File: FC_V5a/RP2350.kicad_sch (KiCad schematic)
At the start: 29 parts, among them SW4 SW_Push, U11 W25Q128JVS, U18 RP2350_60QFN, Y1 ABM8-272-T3

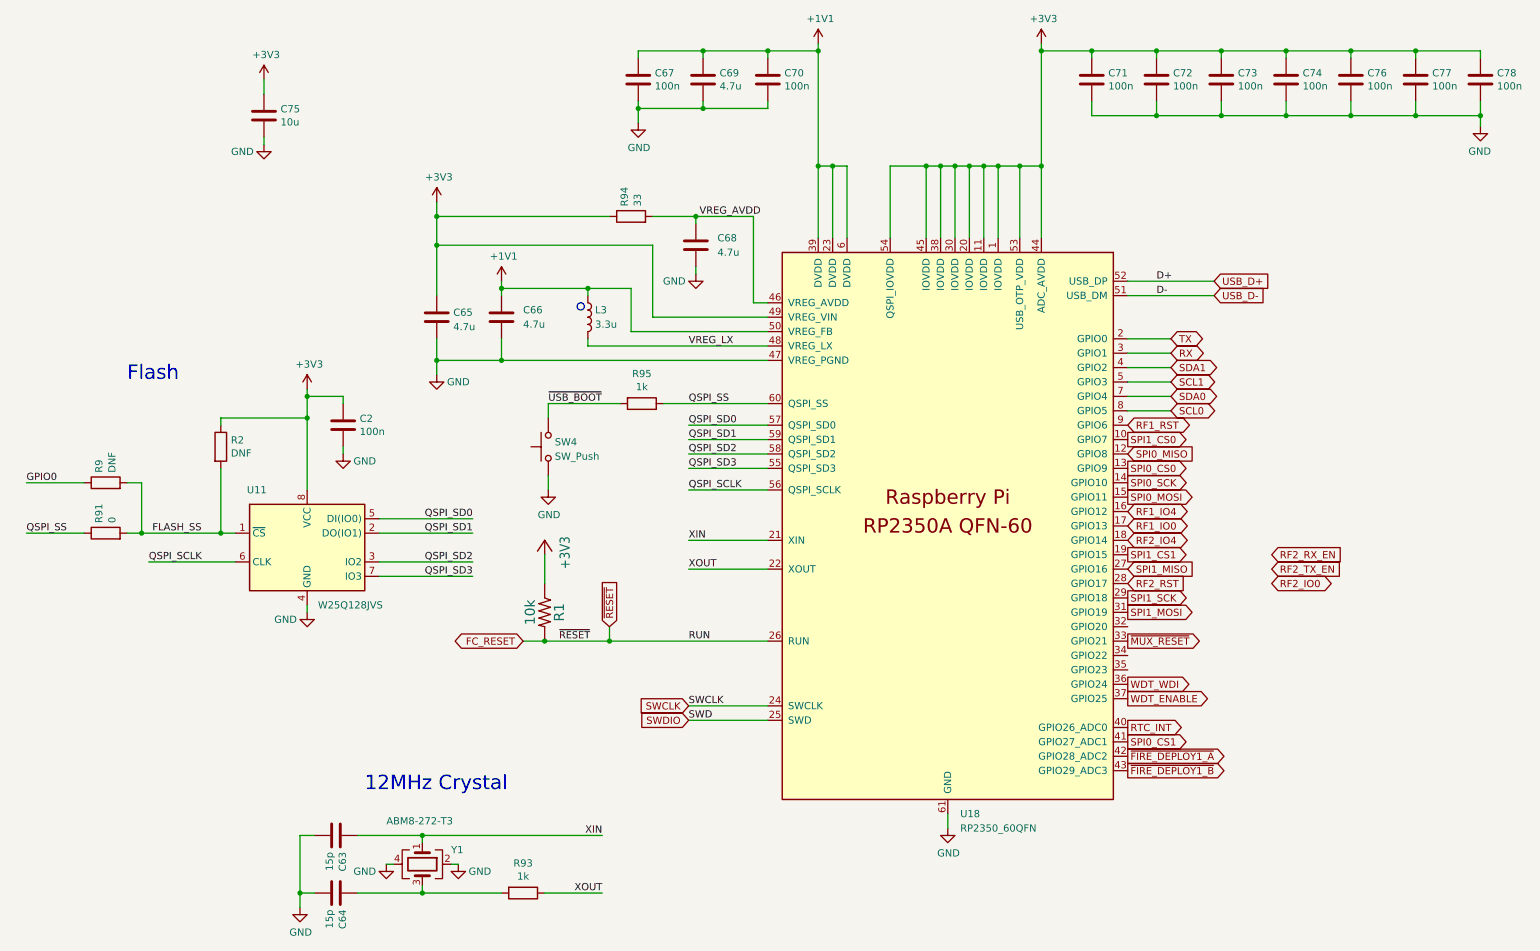
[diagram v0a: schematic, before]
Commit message: Initial V5a Layout Complete
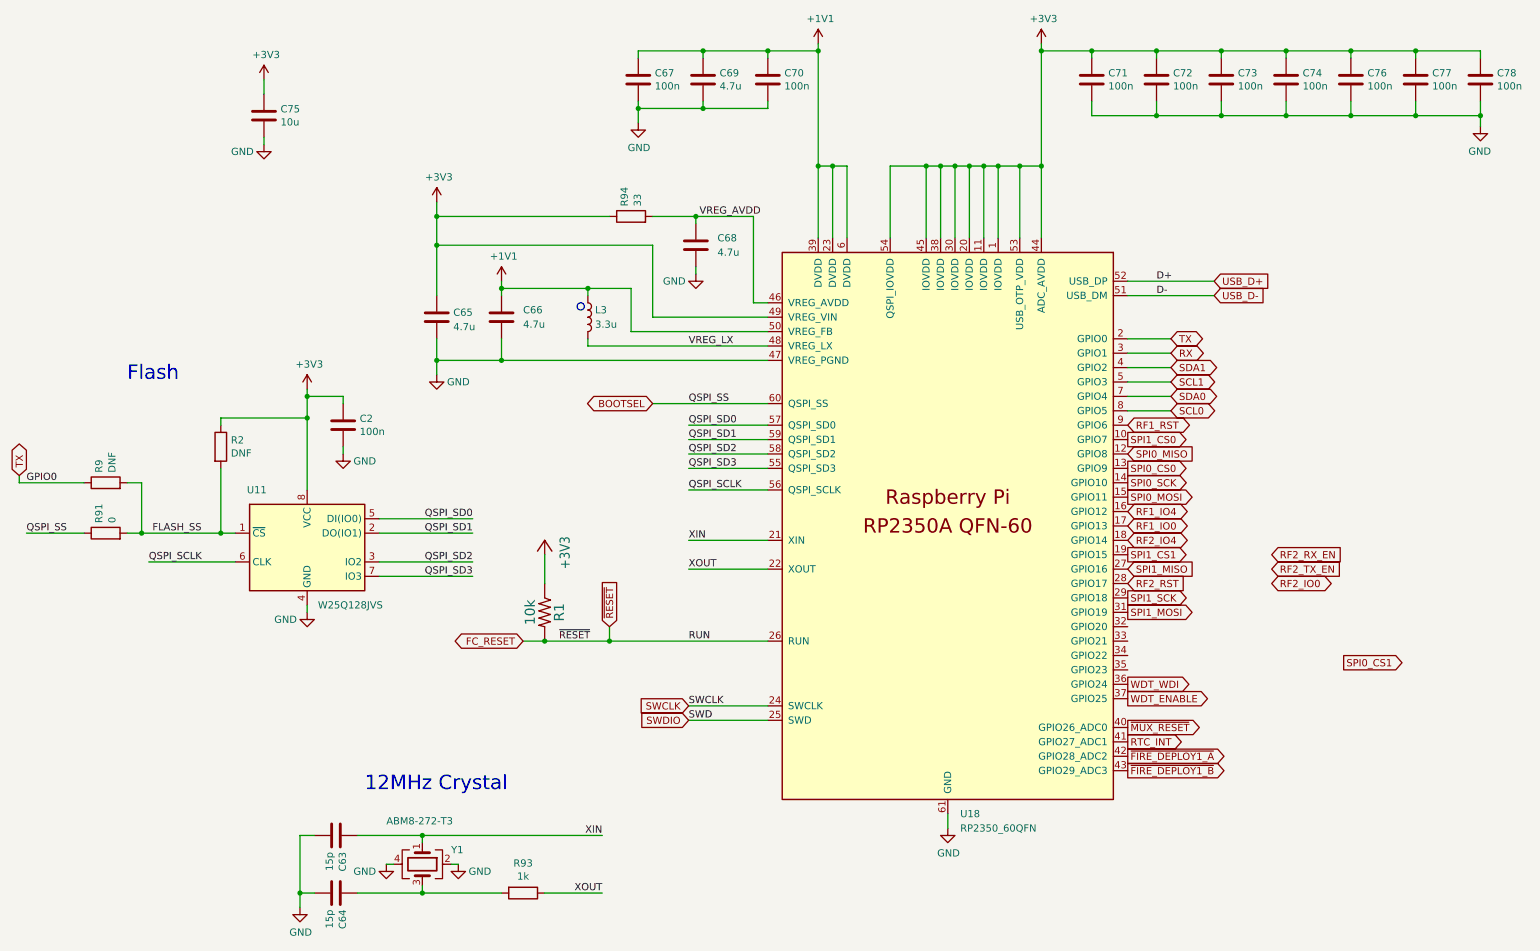
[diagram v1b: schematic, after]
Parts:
- removed R95: 1k, Resistor_SMD:R_0402_1005Metric, symbol Device:R
- removed SW4: SW_Push, Button_Switch_SMD:SW_Push_1P1T_NO_Vertical_Wuerth_434133025816, symbol Switch:SW_Push
- U11: footprint Package_SO:SOIC-8_5.23x5.23mm_P1.27mm -> Package_SO:SOIC-8_5.3x5.3mm_P1.27mm
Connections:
- net GPIO0 is gone; now on net TX: R9.1
- net RTC_INT: now also U18.41 (GPIO27_ADC1); no longer U18.40 (GPIO26_ADC0)
- net SPI0_CS1: no longer U18.41 (GPIO27_ADC1)
- net ~{MUX_RESET}: now also U18.40 (GPIO26_ADC0); no longer U18.33 (GPIO21)
- net QSPI_SS renamed BOOTSEL

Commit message: Initial DRC Errors Cleaned Up
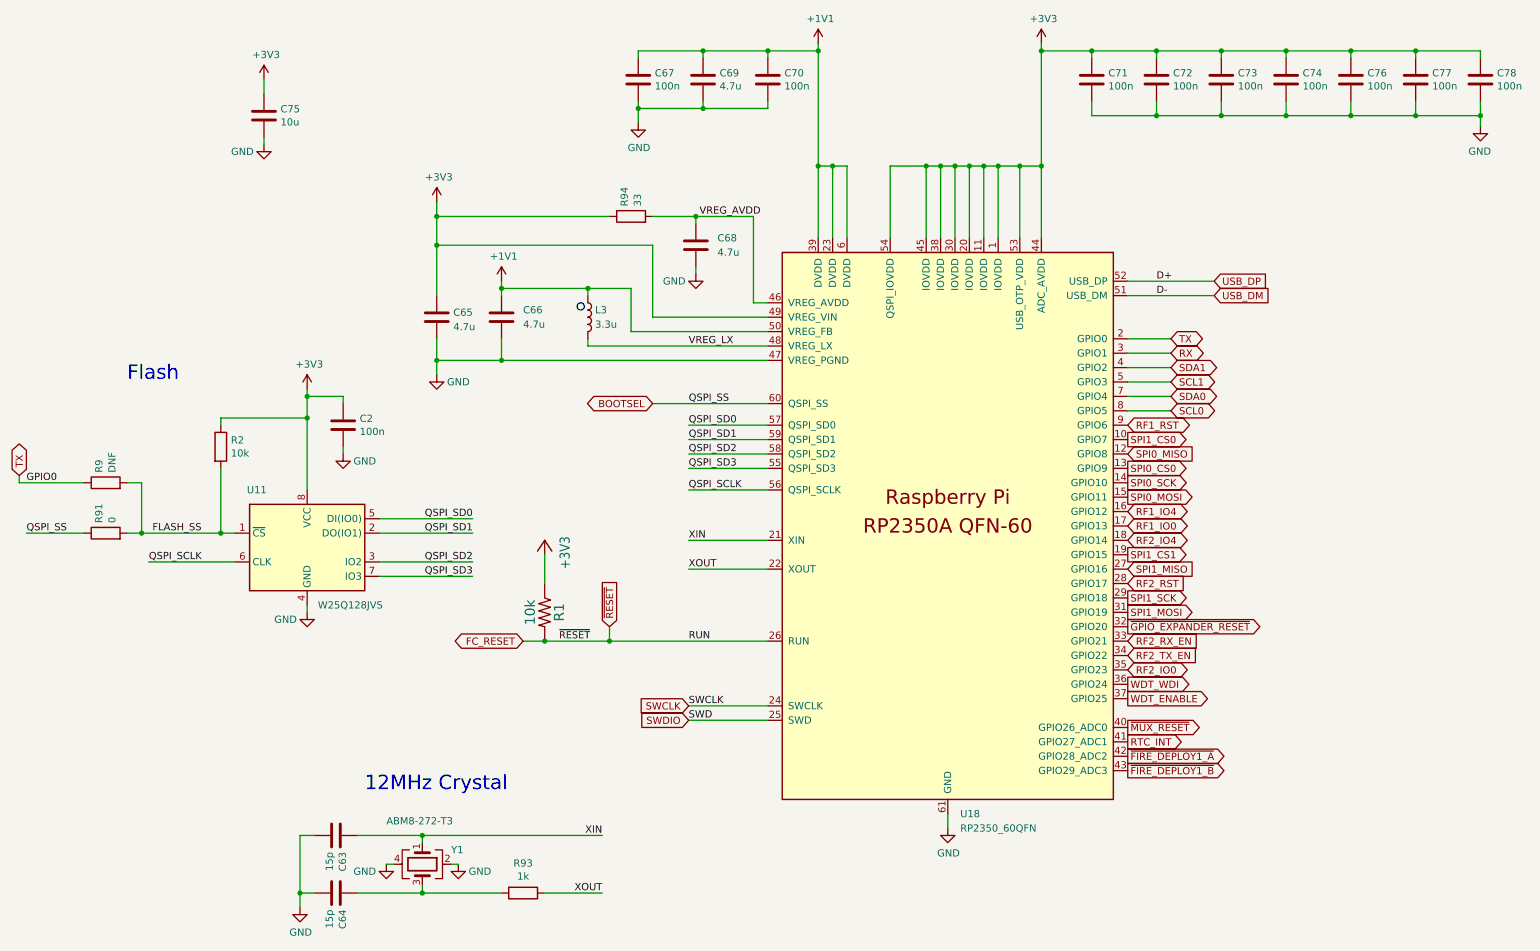
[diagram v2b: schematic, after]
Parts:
- R2: value DNF -> 10k
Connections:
- net RF2_IO0: now also U18.35 (GPIO23)
- net RF2_RX_EN: now also U18.33 (GPIO21)
- net RF2_TX_EN: now also U18.34 (GPIO22)
- net ~{GPIO_EXPANDER_RESET}: now reaches U18.32 (GPIO20)
- net USB_D+ renamed USB_DP
- net USB_D- renamed USB_DM
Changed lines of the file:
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@@
+		)
+	)
+	(global_label "~{GPIO_EXPANDER_RESET}"
+		(shape output)
+		(at 209.55 123.19 0)
+		(fields_autoplaced yes)
+		(effects
+			(font
+				(size 1.27 1.27)
+			)
+			(justify left)
+		)
+		(property "Intersheetrefs" "${INTERSHEET_REFS}"
+			(at 234.4274 123.19 0)
+			(effects
+				(font
+					(size 1.27 1.27)
+				)
+				(justify left)
+				(hide yes)
+			)
+		)
+	)
+	(global_label "RF2_TX_EN"
+		(shape input)
+		(at 209.55 128.27 0)
+		(fields_autoplaced yes)
+		(effects
+			(font
+				(size 1.27 1.27)
+			)
+			(justify left)
+		)
+		(property "Intersheetrefs" "${INTERSHEET_REFS}"
+			(at 222.6951 128.27 0)
+			(effects
+				(font
+					(size 1.27 1.27)
+				)
+				(justify left)
+				(hide yes)
+			)
 		)
 	)
@@
 		(property "Intersheetrefs" "${INTERSHEET_REFS}"
 			(at 221.327 107.95 0)
+			(effects
+				(font
+					(size 1.27 1.27)
+				)
+				(justify left)
+				(hide yes)
+			)
+		)
+	)
+	(global_label "RF2_IO0"
+		(shape bidirectional)
+		(at 209.55 130.81 0)
+		(fields_autoplaced yes)
+		(effects
+			(font
+				(size 1.27 1.27)
+			)
+			(justify left)
+		)
+		(property "Intersheetrefs" "${INTERSHEET_REFS}"
+			(at 221.327 130.81 0)
 			(effects
 				(font
@@
 		)
 	)
-	(global_label "RF2_IO0"
-		(shape bidirectional)
-		(at 234.95 115.57 0)
-		(fields_autoplaced yes)
-		(effects
-			(font
-				(size 1.27 1.27)
-			)
-			(justify left)
-		)
-		(property "Intersheetrefs" "${INTERSHEET_REFS}"
-			(at 246.727 115.57 0)
-			(effects
-				(font
-					(size 1.27 1.27)
-				)
-				(justify left)
-				(hide yes)
-			)
-		)
-	)
 	(global_label "~{FIRE_DEPLOY1_A}"
 		(shape output)
@@
 		)
 	)
-	(global_label "USB_D-"
+	(global_label "USB_DM"
 		(shape input)
 		(at 224.79 64.77 0)
@@
 		)
 		(property "Intersheetrefs" "${INTERSHEET_REFS}"
-			(at 235.3952 64.77 0)
+			(at 235.2742 64.77 0)
 			(effects
 				(font
@@
 		)
 	)
-	(global_label "RF2_TX_EN"
-		(shape input)
-		(at 234.95 113.03 0)
-		(fields_autoplaced yes)
-		(effects
-			(font
-				(size 1.27 1.27)
-			)
-			(justify left)
-		)
-		(property "Intersheetrefs" "${INTERSHEET_REFS}"
-			(at 248.0951 113.03 0)
-			(effects
-				(font
-					(size 1.27 1.27)
-				)
-				(justify left)
-				(hide yes)
-			)
-		)
-	)
 	(global_label "SWDIO"
 		(shape input)
@@
 		)
 	)
-	(global_label "SPI0_CS1"
-		(shape output)
-		(at 247.65 129.54 0)
-		(fields_autoplaced yes)
-		(effects
-			(font
-				(size 1.27 1.27)
-			)
-			(justify left)
-		)
-		(property "Intersheetrefs" "${INTERSHEET_REFS}"
-			(at 259.5856 129.54 0)
-			(effects
-				(font
-					(size 1.27 1.27)
-				)
-				(justify left)
-				(hide yes)
-			)
-		)
-	)
 	(global_label "FC_RESET"
 		(shape bidirectional)
@@
 		(property "Intersheetrefs" "${INTERSHEET_REFS}"
 			(at 224.3002 85.0106 0)
+			(effects
+				(font
+					(size 1.27 1.27)
+				)
+				(justify left)
+				(hide yes)
+			)
+		)
+	)
+	(global_label "RF1_IO4"
+		(shape bidirectional)
+		(at 209.55 102.87 0)
+		(fields_autoplaced yes)
+		(effects
+			(font
+				(size 1.27 1.27)
+			)
+			(justify left)
+		)
+		(property "Intersheetrefs" "${INTERSHEET_REFS}"
+			(at 139.7 -39.37 0)
+			(effects
+				(font
+					(size 1.27 1.27)
+				)
+				(hide yes)
+			)
+		)
+	)
+	(global_label "SPI1_SCK"
+		(shape output)
+		(at 209.55 118.11 0)
+		(fields_autoplaced yes)
+		(effects
+			(font
+				(size 1.27 1.27)
+			)
+			(justify left)
+		)
+		(property "Intersheetrefs" "${INTERSHEET_REFS}"
+			(at 221.5461 118.11 0)
+			(effects
+				(font
+					(size 1.27 1.27)
+				)
+				(justify left)
+				(hide yes)
+			)
+		)
+	)
+	(global_label "WDT_ENABLE"
+		(shape output)
+		(at 209.55 135.89 0)
+		(fields_autoplaced yes)
+		(effects
+			(font
+				(size 1.27 1.27)
+			)
+			(justify left)
+		)
+		(property "Intersheetrefs" "${INTERSHEET_REFS}"
+			(at 224.207 135.89 0)
+			(effects
+				(font
+					(size 1.27 1.27)
+				)
+				(justify left)
+				(hide yes)
+			)
+		)
+	)
+	(global_label "TX"
+		(shape bidirectional)
+		(at 217.17 72.39 0)
+		(fields_autoplaced yes)
+		(effects
+			(font
+				(size 1.27 1.27)
+			)
+			(justify left)
+		)
+		(property "Intersheetrefs" "${INTERSHEET_REFS}"
+			(at 223.3642 72.39 0)
 			(effects
 				(font
@@
 	(global_label "RF2_RX_EN"
 		(shape input)
-		(at 234.95 110.49 0)
-		(fields_autoplaced yes)
-		(effects
-			(font
-				(size 1.27 1.27)
-			)
-			(justify left)
-		)
-		(property "Intersheetrefs" "${INTERSHEET_REFS}"
-			(at 248.3975 110.49 0)
-			(effects
-				(font
-					(size 1.27 1.27)
-				)
-				(justify left)
-				(hide yes)
-			)
-		)
-	)
-	(global_label "RF1_IO4"
-		(shape bidirectional)
-		(at 209.55 102.87 0)
-		(fields_autoplaced yes)
-		(effects
-			(font
-				(size 1.27 1.27)
-			)
-			(justify left)
-		)
-		(property "Intersheetrefs" "${INTERSHEET_REFS}"
-			(at 139.7 -39.37 0)
-			(effects
-				(font
-					(size 1.27 1.27)
-				)
-				(hide yes)
-			)
-		)
-	)
-	(global_label "SPI1_SCK"
-		(shape output)
-		(at 209.55 118.11 0)
-		(fields_autoplaced yes)
-		(effects
-			(font
-				(size 1.27 1.27)
-			)
-			(justify left)
-		)
-		(property "Intersheetrefs" "${INTERSHEET_REFS}"
-			(at 221.5461 118.11 0)
-			(effects
-				(font
-					(size 1.27 1.27)
-				)
-				(justify left)
-				(hide yes)
-			)
-		)
-	)
-	(global_label "WDT_ENABLE"
-		(shape output)
-		(at 209.55 135.89 0)
-		(fields_autoplaced yes)
-		(effects
-			(font
-				(size 1.27 1.27)
-			)
-			(justify left)
-		)
-		(property "Intersheetrefs" "${INTERSHEET_REFS}"
-			(at 224.207 135.89 0)
-			(effects
-				(font
-					(size 1.27 1.27)
-				)
-				(justify left)
-				(hide yes)
-			)
-		)
-	)
-	(global_label "TX"
-		(shape bidirectional)
-		(at 217.17 72.39 0)
-		(fields_autoplaced yes)
-		(effects
-			(font
-				(size 1.27 1.27)
-			)
-			(justify left)
-		)
-		(property "Intersheetrefs" "${INTERSHEET_REFS}"
-			(at 223.3642 72.39 0)
+		(at 209.55 125.73 0)
+		(fields_autoplaced yes)
+		(effects
+			(font
+				(size 1.27 1.27)
+			)
+			(justify left)
+		)
+		(property "Intersheetrefs" "${INTERSHEET_REFS}"
+			(at 222.9975 125.73 0)
 			(effects
 				(font
@@
 		)
 	)
-	(global_label "USB_D+"
+	(global_label "USB_DP"
 		(shape input)
 		(at 224.79 62.23 0)
@@
 		)
 		(property "Intersheetrefs" "${INTERSHEET_REFS}"
-			(at 235.3952 62.23 0)
+			(at 235.0928 62.23 0)
 			(effects
 				(font
@@
 			)
 		)
-		(property "Value" "DNF"
+		(property "Value" "10k"
 			(at 51.308 92.583 0)
 			(effects
